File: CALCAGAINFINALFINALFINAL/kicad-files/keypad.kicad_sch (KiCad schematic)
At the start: 101 parts, among them SW100 SW_SPST, SW101 SW_SPST, SW102 SW_SPST, SW49 SW_SPST, SW52 SW_SPST, SW55 SW_SPST, SW56 SW_SPST, SW57 SW_SPST, SW58 SW_SPST, SW59 SW_SPST, SW60 SW_SPST, SW61 SW_SPST, SW62 SW_SPST, SW63 SW_SPST, SW64 SW_SPST, SW65 SW_SPST, SW66 SW_SPST, SW67 SW_SPST, SW68 SW_SPST, SW69 SW_SPST, SW70 SW_SPST, SW71 SW_SPST, SW72 SW_SPST, SW73 SW_SPST, SW74 SW_SPST, SW75 SW_SPST, SW76 SW_SPST, SW77 SW_SPST, SW78 SW_SPST, SW79 SW_SPST, SW80 SW_SPST, SW81 SW_SPST, SW82 SW_SPST, SW83 SW_SPST, SW84 SW_SPST, SW85 SW_SPST, SW86 SW_SPST, SW87 SW_SPST, SW88 SW_SPST, SW89 SW_SPST, SW90 SW_SPST, SW91 SW_SPST, SW92 SW_SPST, SW93 SW_SPST, SW94 SW_SPST, SW95 SW_SPST, SW96 SW_SPST, SW97 SW_SPST, SW98 SW_SPST, SW99 SW_SPST, U7 TCA9535DBR

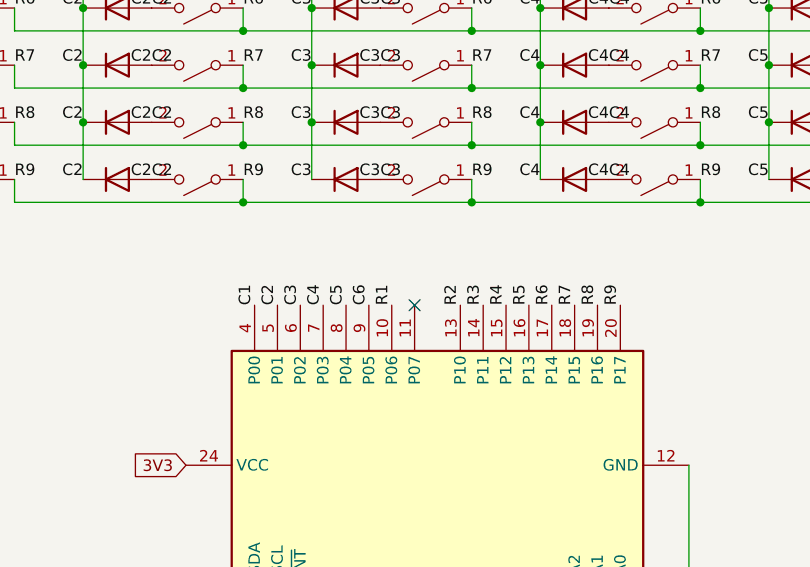
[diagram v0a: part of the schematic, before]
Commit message: Turns out my whole power thing was absolutely retarded i should REALLY stop relying on gemini its actually retarded as fuh. Ima start js rawdogging it w forums and reddit. once its functional ima order it. i gota remember there no deadline better do it right the first time.
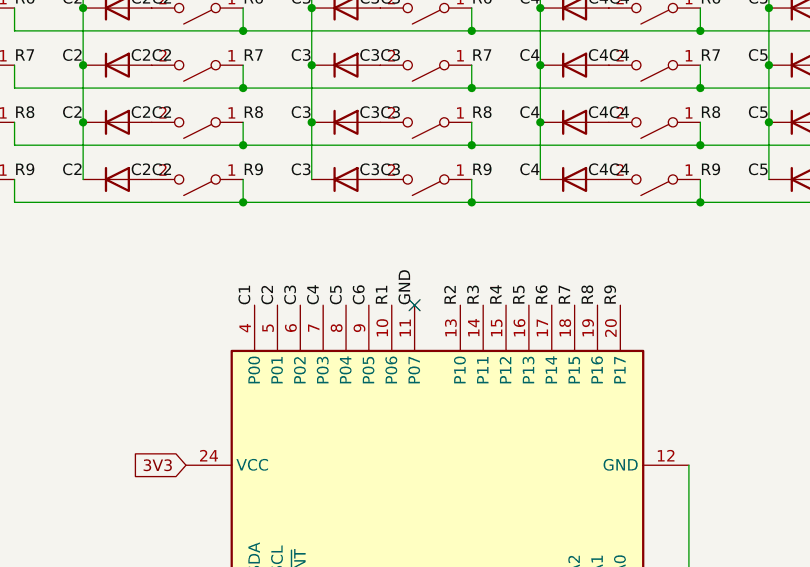
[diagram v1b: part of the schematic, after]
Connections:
- net GND: now also U7.11 (P07)
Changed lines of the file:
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@@
+		)
+	)
+	(label "GND"
+		(at 134.62 112.014 90)
+		(effects
+			(font
+				(size 1.27 1.27)
+			)
+			(justify left bottom)
 		)
 	)
